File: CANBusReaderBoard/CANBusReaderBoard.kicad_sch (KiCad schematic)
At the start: 31 parts, among them J2 3xRJ45V, J4 Jack-DC, J5 Terminate CAN, SW1 SW_DIP_x01, U1 Pico, U3 MCP2515-E{slash}P, U4 NCV5501DT50RKG, U5 MCP2562-E-P, Y1 Crystal 20Mhz

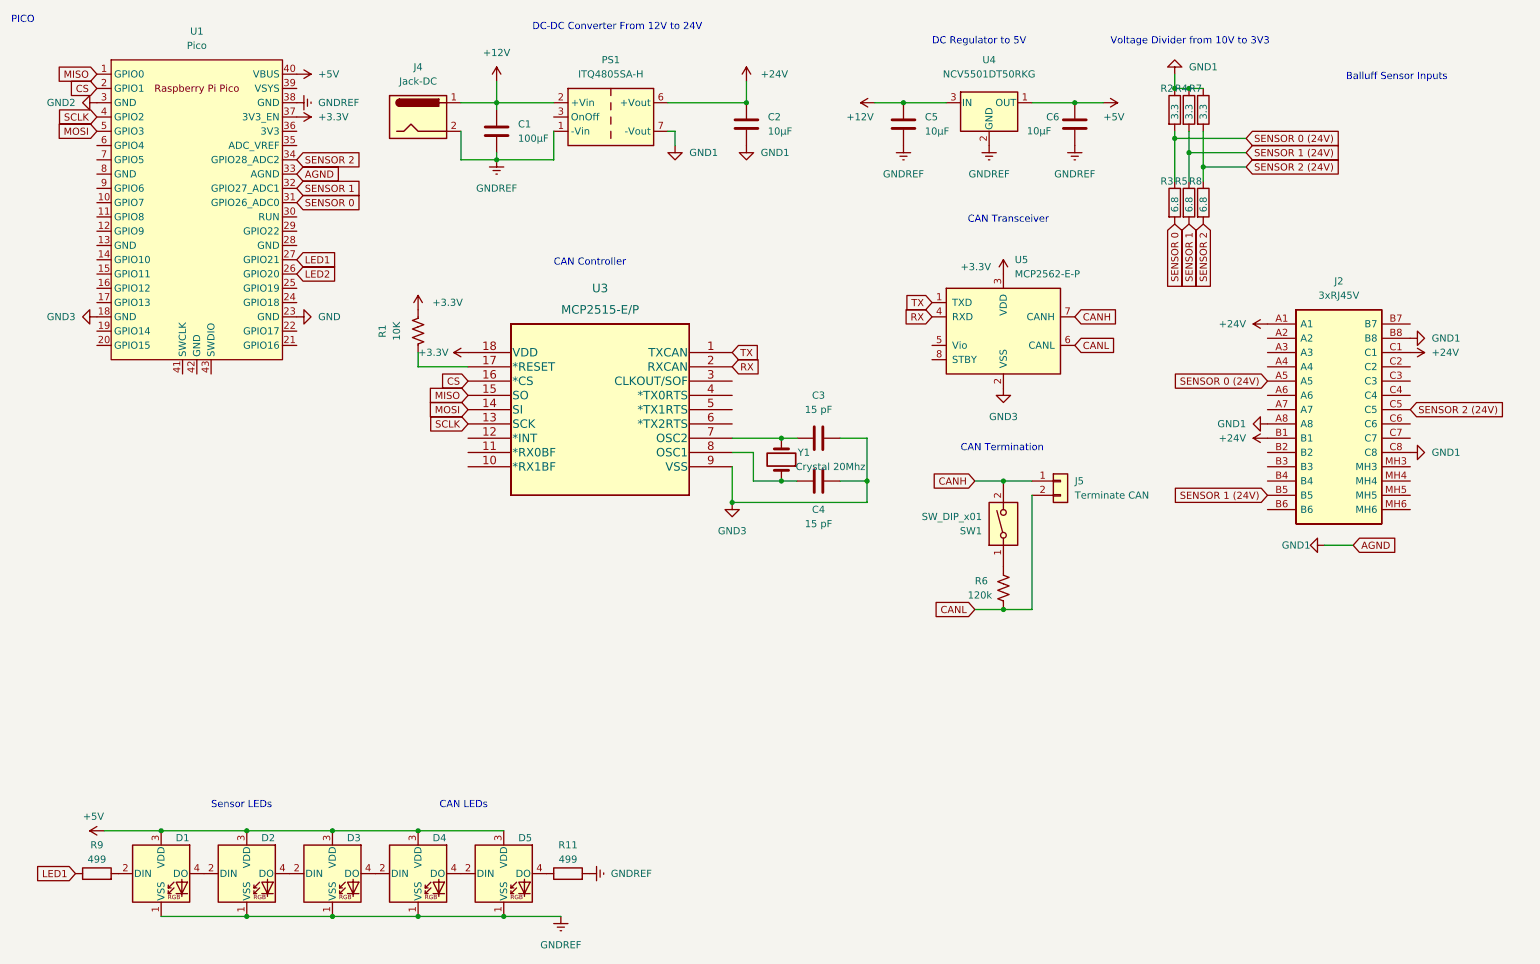
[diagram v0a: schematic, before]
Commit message: code init
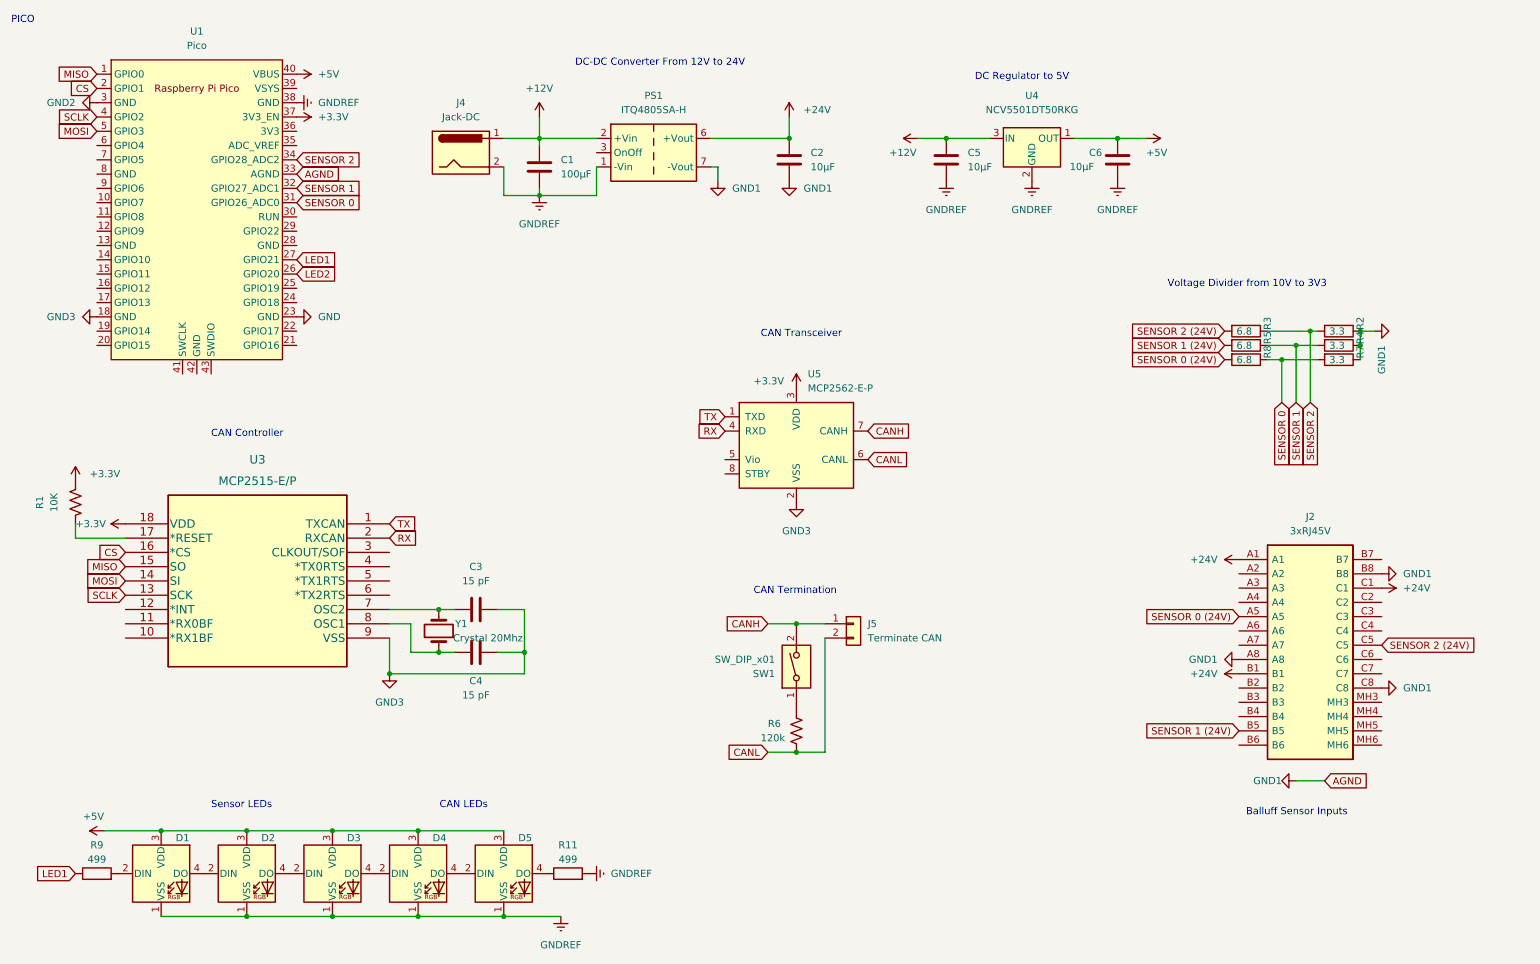
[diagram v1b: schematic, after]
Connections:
- net SENSOR 0: now also R7.2, R8.1; no longer R3.2
- net SENSOR 0 (24V): now also R8.2; no longer R2.2, R3.1
- net SENSOR 1: now also R4.2, R5.1; no longer R5.2
- net SENSOR 1 (24V): now also R5.2; no longer R4.2, R5.1
- net SENSOR 2: now also R2.2, R3.1; no longer R8.2
- net SENSOR 2 (24V): now also R3.2; no longer R7.2, R8.1
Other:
- moved on the sheet: C1, C2, C3, C4, C5, C6, J2, J4, J5, PS1, R1, R2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
